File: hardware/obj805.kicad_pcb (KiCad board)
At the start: 2 copper layers, 38 parts, among them J0 Conn_with_rapi, U1 l293d

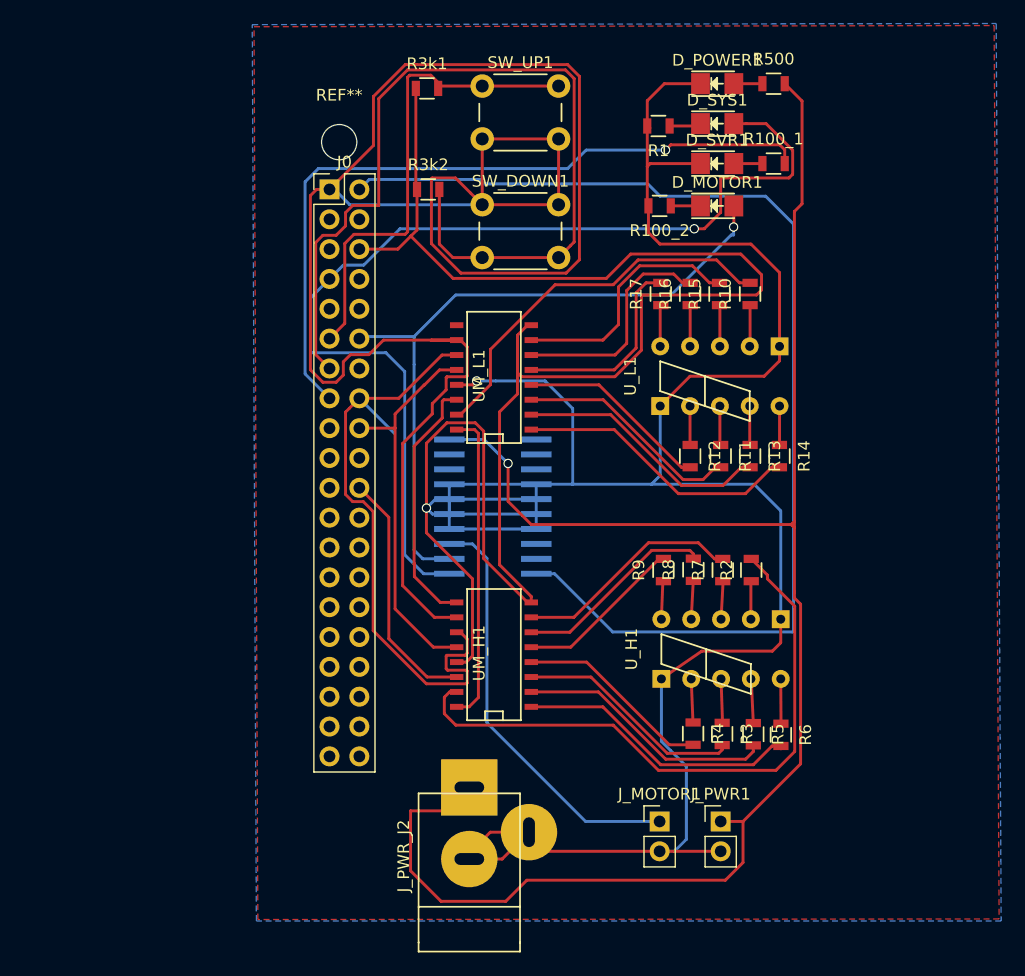
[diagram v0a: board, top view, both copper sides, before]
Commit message: update;
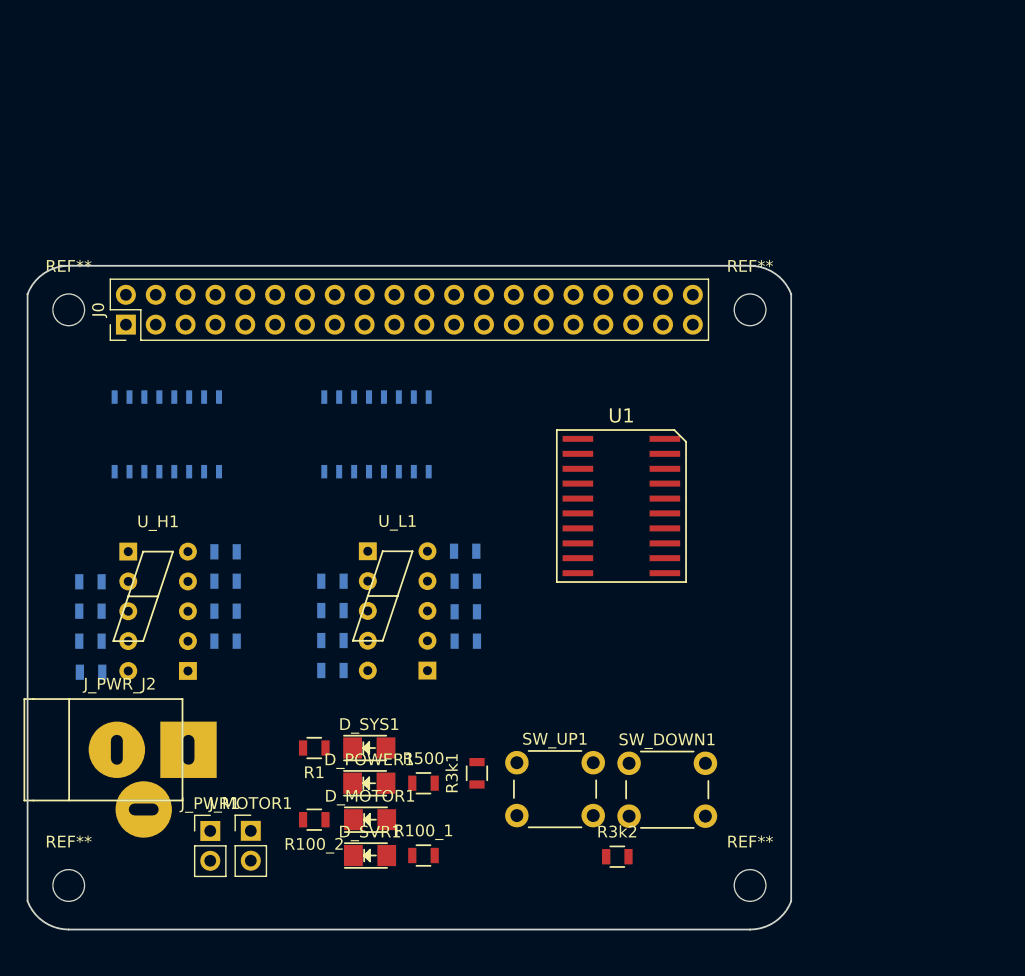
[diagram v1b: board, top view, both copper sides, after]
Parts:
- removed the REF** at (47.0, 28.0)
- added REF**: MountingHole_2.7mm_M2.5, Mounting_Holes:MountingHole_2.7mm_M2.5, F.Cu at (24.0, 91.2)
- added REF**: MountingHole_2.7mm_M2.5, Mounting_Holes:MountingHole_2.7mm_M2.5, F.Cu at (82.0, 91.2)
- added REF**: MountingHole_2.7mm_M2.5, Mounting_Holes:MountingHole_2.7mm_M2.5, F.Cu at (82.0, 42.2)
- added REF**: MountingHole_2.7mm_M2.5, Mounting_Holes:MountingHole_2.7mm_M2.5, F.Cu at (24.0, 42.2)
- R10, R11, R12, R13, R14, R15, R16, R17, R2, R3, R4, R5, R6, R7, R8, R9, UM_H1, UM_L1: moved to B.Cu
- U1: moved to F.Cu
- moved R500 66.6 mm to (54.2, 82.5)
- moved D_POWER1 66.5 mm to (49.6, 82.5)
- moved R100_1 66.0 mm to (54.2, 88.7)
- moved D_SVR1 65.9 mm to (49.6, 88.7)
- moved D_SYS1 60.8 mm to (49.6, 79.5)
- moved R1 60.5 mm to (44.9, 79.5)
- moved D_MOTOR1 60.0 mm to (49.6, 85.7)
- moved R100_2 60.0 mm to (44.9, 85.7)
- moved R3k2 59.0 mm to (70.7, 88.8)
- moved R6 59.0 mm to (25.9, 73.1), turned to 180 degrees
- moved R3k1 58.5 mm to (58.8, 81.7), turned to 90 degrees
- moved SW_UP1 57.7 mm to (62.1, 80.8)
- moved R5 57.0 mm to (25.9, 70.5), turned to 180 degrees
- moved R3 54.8 mm to (25.9, 67.9), turned to 180 degrees
- moved R4 52.9 mm to (25.9, 65.4), turned to 180 degrees
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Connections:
- D_POWER1 pad 1: GND -> Net-(D_POWER1-Pad1)
- D_SVR1 pad 1: GND -> Net-(D_POWER1-Pad1)
- J0 pad 6: GND -> Net-(D_POWER1-Pad1)
- J_MOTOR1 pad 2: GND -> Net-(D_POWER1-Pad1)
- J_PWR1 pad 2: GND -> Net-(D_POWER1-Pad1)
- J_PWR_J2 pad 2: GND -> Net-(D_POWER1-Pad1)
- J_PWR_J2 pad 3: GND -> Net-(D_POWER1-Pad1)
- R1 pad 2: GND -> Net-(D_POWER1-Pad1)
- R100_2 pad 2: GND -> Net-(D_POWER1-Pad1)
- R3k1 pad 1: GND -> Net-(D_POWER1-Pad1)
- R3k2 pad 1: GND -> Net-(D_POWER1-Pad1)
- U1 pad 14: GND -> Net-(D_POWER1-Pad1)
- U1 pad 15: GND -> Net-(D_POWER1-Pad1)
- U1 pad 16: GND -> Net-(D_POWER1-Pad1)
- U1 pad 17: GND -> Net-(D_POWER1-Pad1)
- U1 pad 4: GND -> Net-(D_POWER1-Pad1)
- U1 pad 5: GND -> Net-(D_POWER1-Pad1)
- U1 pad 6: GND -> Net-(D_POWER1-Pad1)
- U1 pad 7: GND -> Net-(D_POWER1-Pad1)
- UM_H1 pad 1: Net-(R6-Pad2) -> Net-(R7-Pad2)
- UM_H1 pad 13: GND -> Net-(D_POWER1-Pad1)
- UM_H1 pad 2: Net-(R5-Pad2) -> Net-(R8-Pad2)
- UM_H1 pad 3: Net-(R3-Pad2) -> Net-(R9-Pad2)
- UM_H1 pad 5: Net-(R9-Pad2) -> Net-(R3-Pad2)
- UM_H1 pad 6: Net-(R8-Pad2) -> Net-(R5-Pad2)
- UM_H1 pad 7: Net-(R7-Pad2) -> Net-(R6-Pad2)
- UM_L1 pad 1: Net-(R14-Pad2) -> Net-(R15-Pad2)
- UM_L1 pad 13: GND -> Net-(D_POWER1-Pad1)
- UM_L1 pad 2: Net-(R13-Pad2) -> Net-(R16-Pad2)
- UM_L1 pad 3: Net-(R11-Pad2) -> Net-(R17-Pad2)
- UM_L1 pad 5: Net-(R17-Pad2) -> Net-(R11-Pad2)
- UM_L1 pad 6: Net-(R16-Pad2) -> Net-(R13-Pad2)
- UM_L1 pad 7: Net-(R15-Pad2) -> Net-(R14-Pad2)
- U_H1 pad 3: GND -> Net-(D_POWER1-Pad1)
- U_H1 pad 8: GND -> Net-(D_POWER1-Pad1)
- U_L1 pad 3: GND -> Net-(D_POWER1-Pad1)
- U_L1 pad 8: GND -> Net-(D_POWER1-Pad1)
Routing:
- net GND: track 363.5 -> 0.00 mm, vias 2 -> 0
- net Net-(J0-Pad1): track 172.0 -> 0.00 mm
- net Net-(J_PWR1-Pad1): track 147.8 -> 0.00 mm, vias 1 -> 0
- net Net-(J0-Pad2): track 97.5 -> 0.00 mm
- net Net-(D_SYS1-Pad2): track 88.4 -> 0.00 mm, vias 1 -> 0
- net Net-(J0-Pad13): track 76.6 -> 0.00 mm
- net Net-(J0-Pad15): track 62.8 -> 0.00 mm, vias 1 -> 0
- net Net-(D_MOTOR1-Pad2): track 59.6 -> 0.00 mm, vias 1 -> 0
- net Net-(J0-Pad16): track 53.9 -> 0.00 mm
- net Net-(R2-Pad2): track 53.1 -> 0.00 mm
- net Net-(J0-Pad11): track 41.3 -> 0.00 mm
- net Net-(J_MOTOR1-Pad1): track 35.9 -> 0.00 mm
- net Net-(J0-Pad18): track 33.3 -> 0.00 mm
- net Net-(R10-Pad2): track 33.0 -> 0.00 mm
- net VCC: track 26.6 -> 0.00 mm
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- removed copper zone on B.Cu, net GND
- removed copper zone on F.Cu, net GND
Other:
- board outline added: 65 x 56.5 mm
- net class Default: trace_width 0.25 -> 0.2
